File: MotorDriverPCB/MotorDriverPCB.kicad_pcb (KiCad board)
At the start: 2 copper layers, 68.5 x 65.5 mm, 10 parts

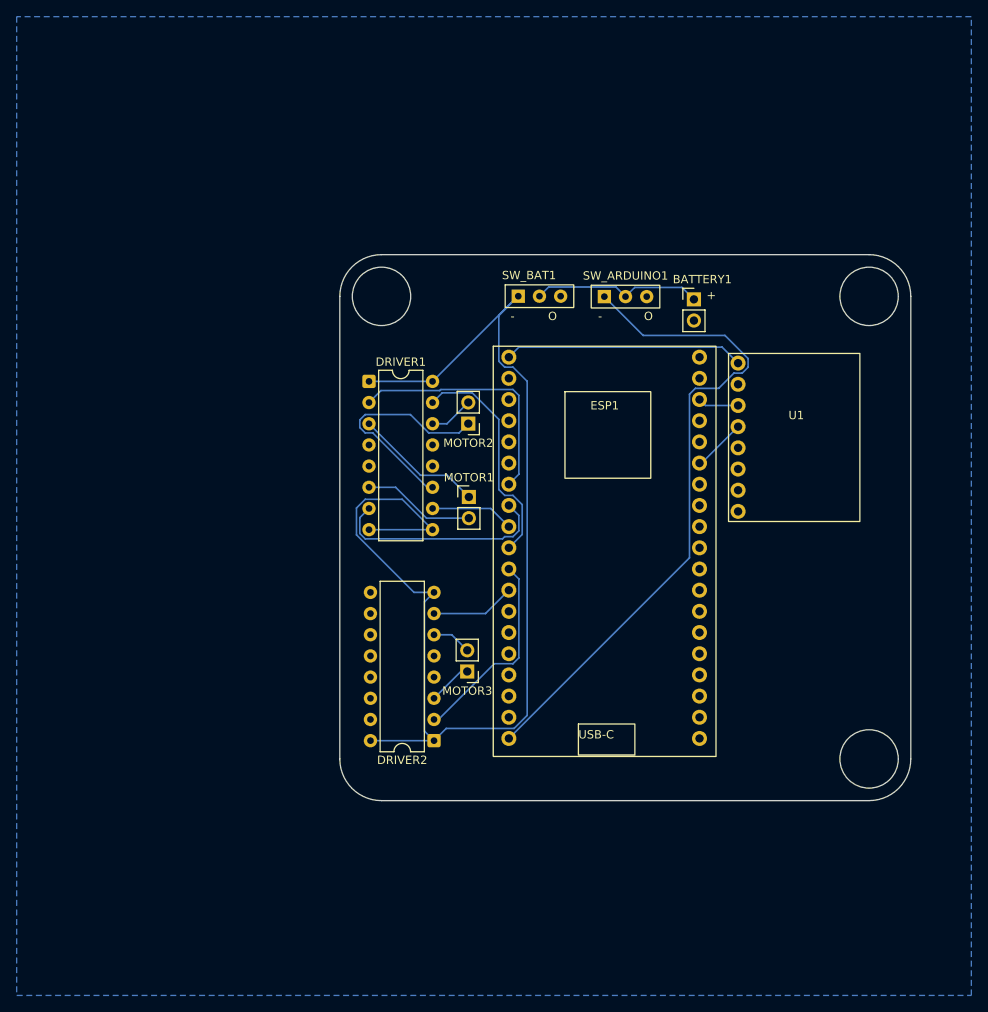
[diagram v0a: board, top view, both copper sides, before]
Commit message: Added Encoders
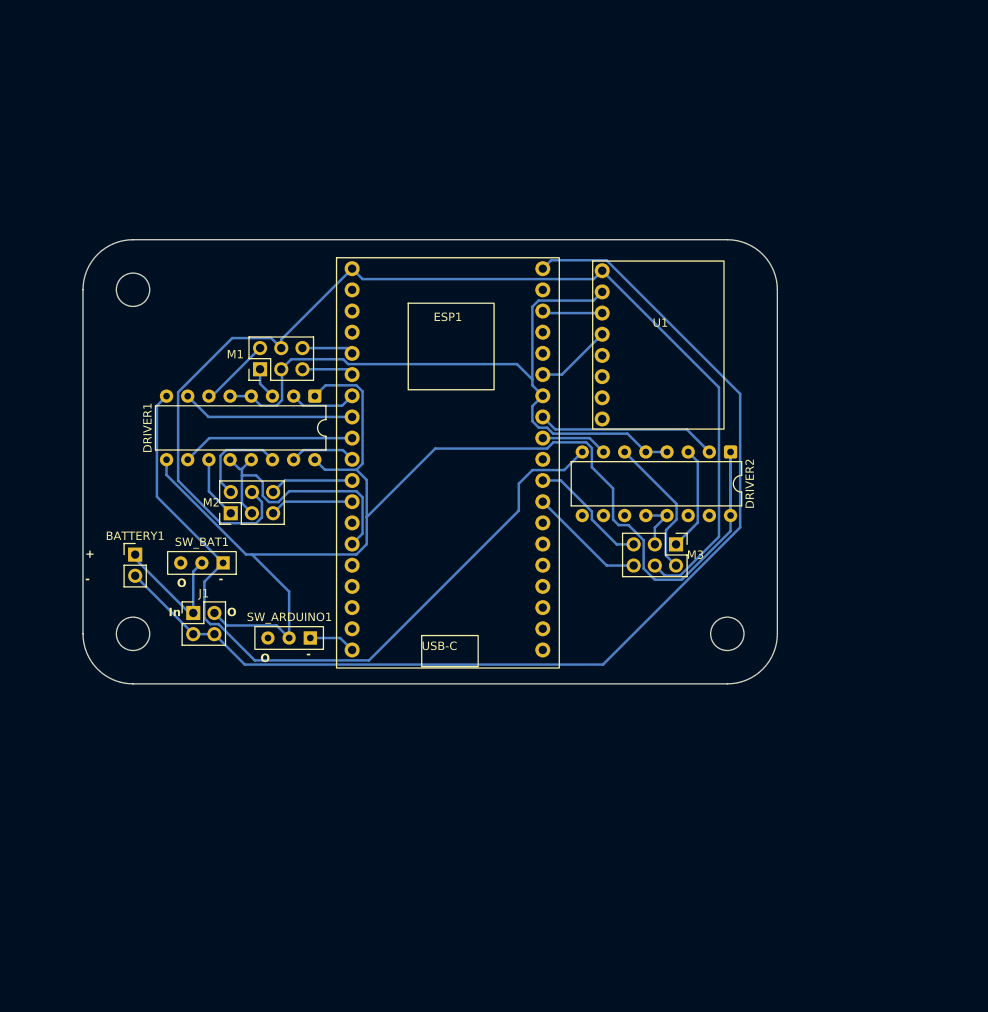
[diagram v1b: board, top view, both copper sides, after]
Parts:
- removed MOTOR1, MOTOR2, MOTOR3: Conn_01x02_Pin, Connector_PinHeader_2.54mm:PinHeader_1x02_P2.54mm_Vertical
- added J1: Conn_02x02_Counter_Clockwise, Connector_PinHeader_2.54mm:PinHeader_2x02_P2.54mm_Vertical, F.Cu at (100.0, 109.5)
- added M1: Conn_02x03_Counter_Clockwise, Headers:Header_02x03, F.Cu at (108.0, 80.3)
- added M2: Conn_02x03_Counter_Clockwise, Headers:Header_02x03, F.Cu at (104.5, 97.5)
- added M3: Conn_02x03_Counter_Clockwise, Headers:Header_02x03, F.Cu at (157.8, 101.3)
- moved BATTERY1 73.7 mm to (93.0, 102.5)
- moved SW_ARDUINO1 57.5 mm to (111.5, 112.5), turned to 180 degrees
- moved SW_BAT1 51.6 mm to (101.0, 103.5), turned to 180 degrees
- moved DRIVER2 49.6 mm to (164.4, 90.2), turned to -90 degrees
- moved ESP1 21.6 mm to (123.4, 99.6)
- moved U1 19.7 mm to (156.0, 75.2)
- moved DRIVER1 6.73 mm to (114.5, 83.5), turned to -90 degrees
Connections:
- DRIVER1 pad 1: /BAT_SW -> /BUCK
- DRIVER1 pad 16: /BAT_SW -> /BUCK
- DRIVER1 pad 9: /BAT_SW -> /BUCK
- DRIVER2 pad 1: /BAT_SW -> /BUCK
- DRIVER2 pad 16: /BAT_SW -> /BUCK
- ESP1 pad P14: /REV3 -> /A2
- ESP1 pad P16: unconnected-(ESP1-GPIO16-PadP16) -> /B3
- ESP1 pad P17: unconnected-(ESP1-GPIO17-PadP17) -> /A3
- ESP1 pad P18: unconnected-(ESP1-GPIO18-PadP18) -> /REV3
- ESP1 pad P19: unconnected-(ESP1-GPIO19-PadP19) -> /FOR3
- ESP1 pad P27: /FOR3 -> /B2
- ESP1 pad P34: unconnected-(ESP1-GPIO34-PadP34) -> /B1
- ESP1 pad P35: unconnected-(ESP1-GPIO35-PadP35) -> /A1
- SW_ARDUINO1 pad 2: /BAT -> /BUCK
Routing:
- net GND: track 0.00 -> 254.0 mm
- net /BUCK: track 0.00 -> 162.8 mm
- net /3V3: track 28.8 -> 133.9 mm
- net /VIN: track 80.0 -> 5.61 mm
- net /BAT_SW: track 148.2 -> 91.0 mm
- net /FOR1: track 30.1 -> 7.99 mm
- net /M2F: track 27.2 -> 7.51 mm
- net /REV2: track 27.6 -> 7.95 mm
- net /A3: track 0.00 -> 14.6 mm
- net /B3: track 0.00 -> 14.1 mm
- net /M3R: track 4.76 -> 17.2 mm
- net /M1F: track 15.6 -> 3.84 mm
- net /FOR2: track 10.1 -> 20.8 mm
- net /B2: track 0.00 -> 10.0 mm
- net /A2: track 0.00 -> 10.0 mm
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- removed copper zone on B.Cu, net GND
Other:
- board size 68.5 x 65.5 mm -> 83.3 x 53.3 mm
- board text added: "In"
